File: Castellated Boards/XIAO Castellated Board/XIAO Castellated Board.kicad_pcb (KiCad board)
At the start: 2 copper layers, 18.5 x 21 mm, 1 part

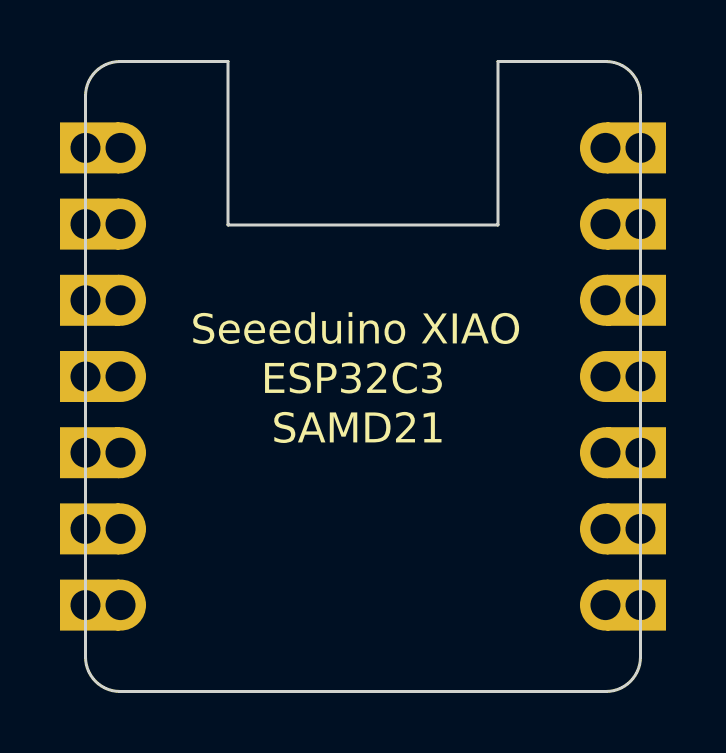
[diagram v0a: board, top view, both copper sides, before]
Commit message: Castellated Boards
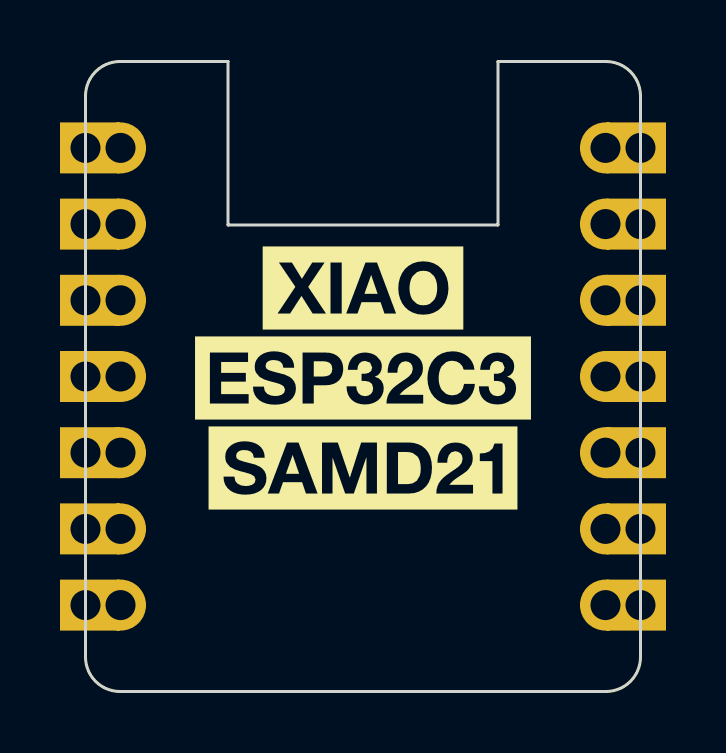
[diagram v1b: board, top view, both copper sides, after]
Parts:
- added kibuzzard-65885ADF: G***, kibuzzard-65885ADF, F.Cu at (100.5, 69.7)
- added kibuzzard-65885AE8: G***, kibuzzard-65885AE8, F.Cu at (100.5, 72.7)
- added kibuzzard-65885AFA: G***, kibuzzard-65885AFA, F.Cu at (100.5, 75.7)
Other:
- board text removed: "ESP32C3"
- board text removed: "SAMD21"
- board text removed: "Seeeduino XIAO"
